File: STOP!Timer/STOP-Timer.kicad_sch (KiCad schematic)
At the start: 18 parts, among them J1 Foot Switch Jack, J4 RJ45, SW1 SW_Push, SW2 SW_Push, SW3 SW_Push, SW4 SW_SPDT, SW5 SW_SPDT

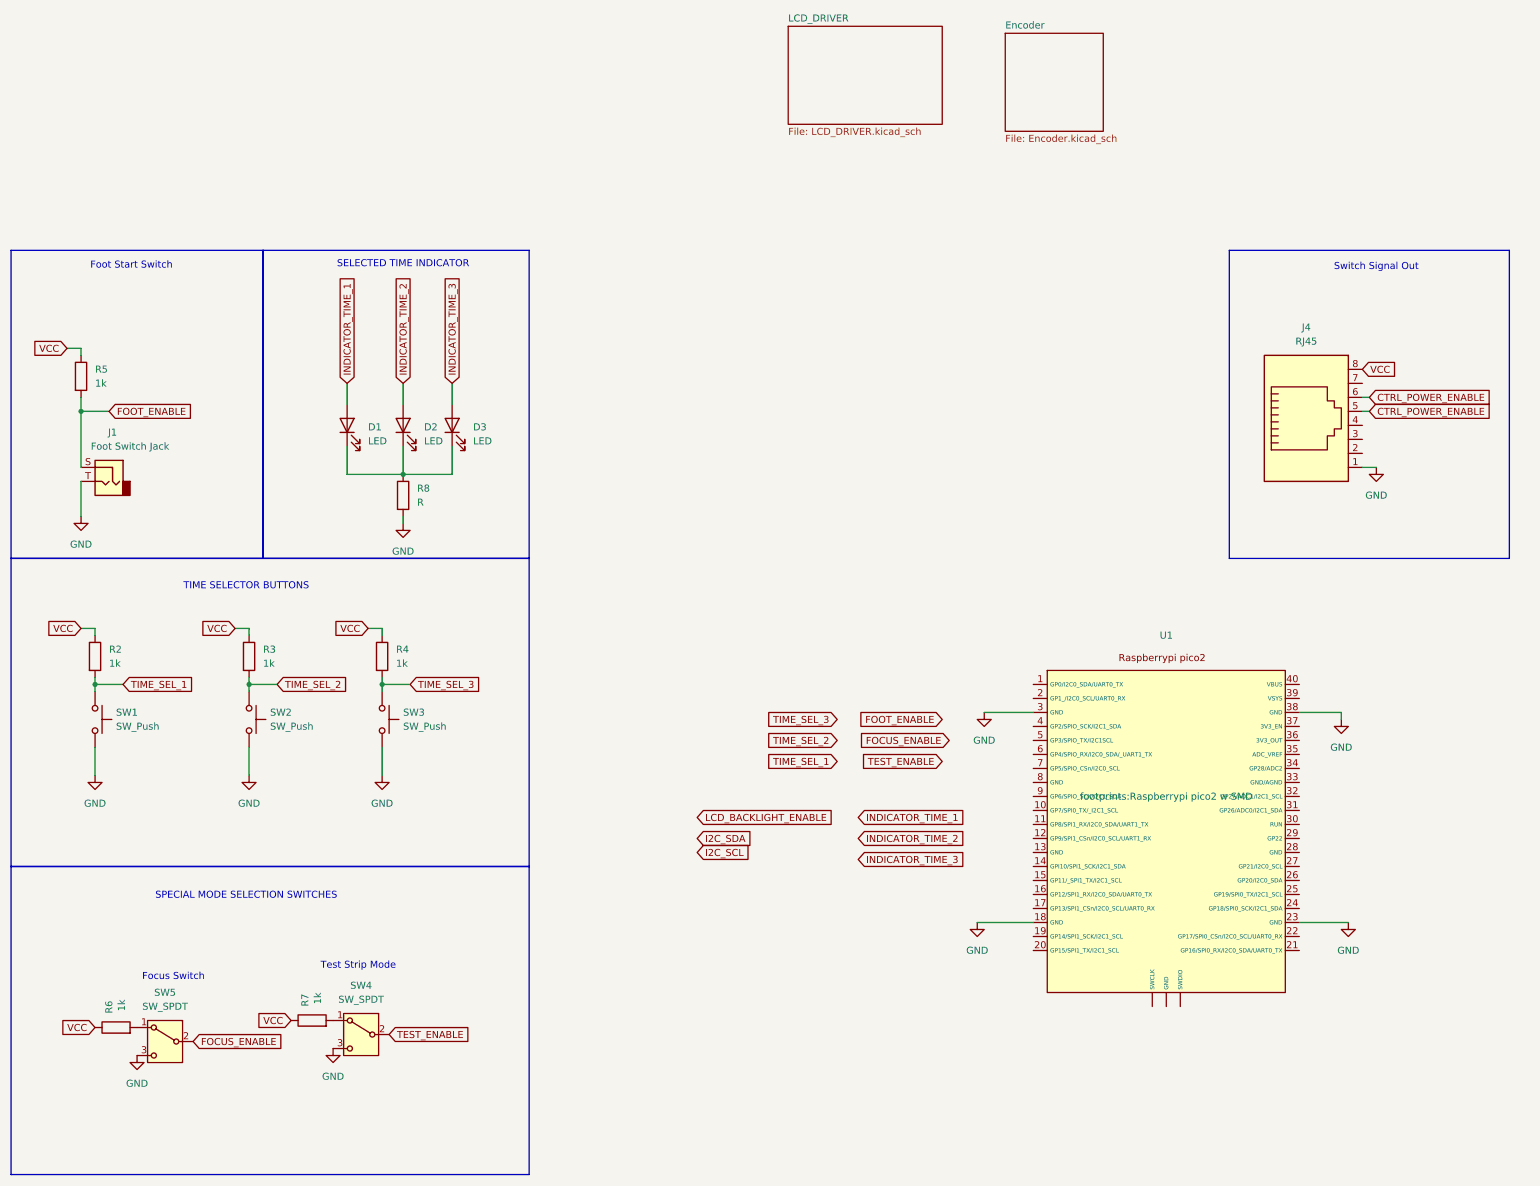
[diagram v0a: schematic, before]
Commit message: Update Schematic
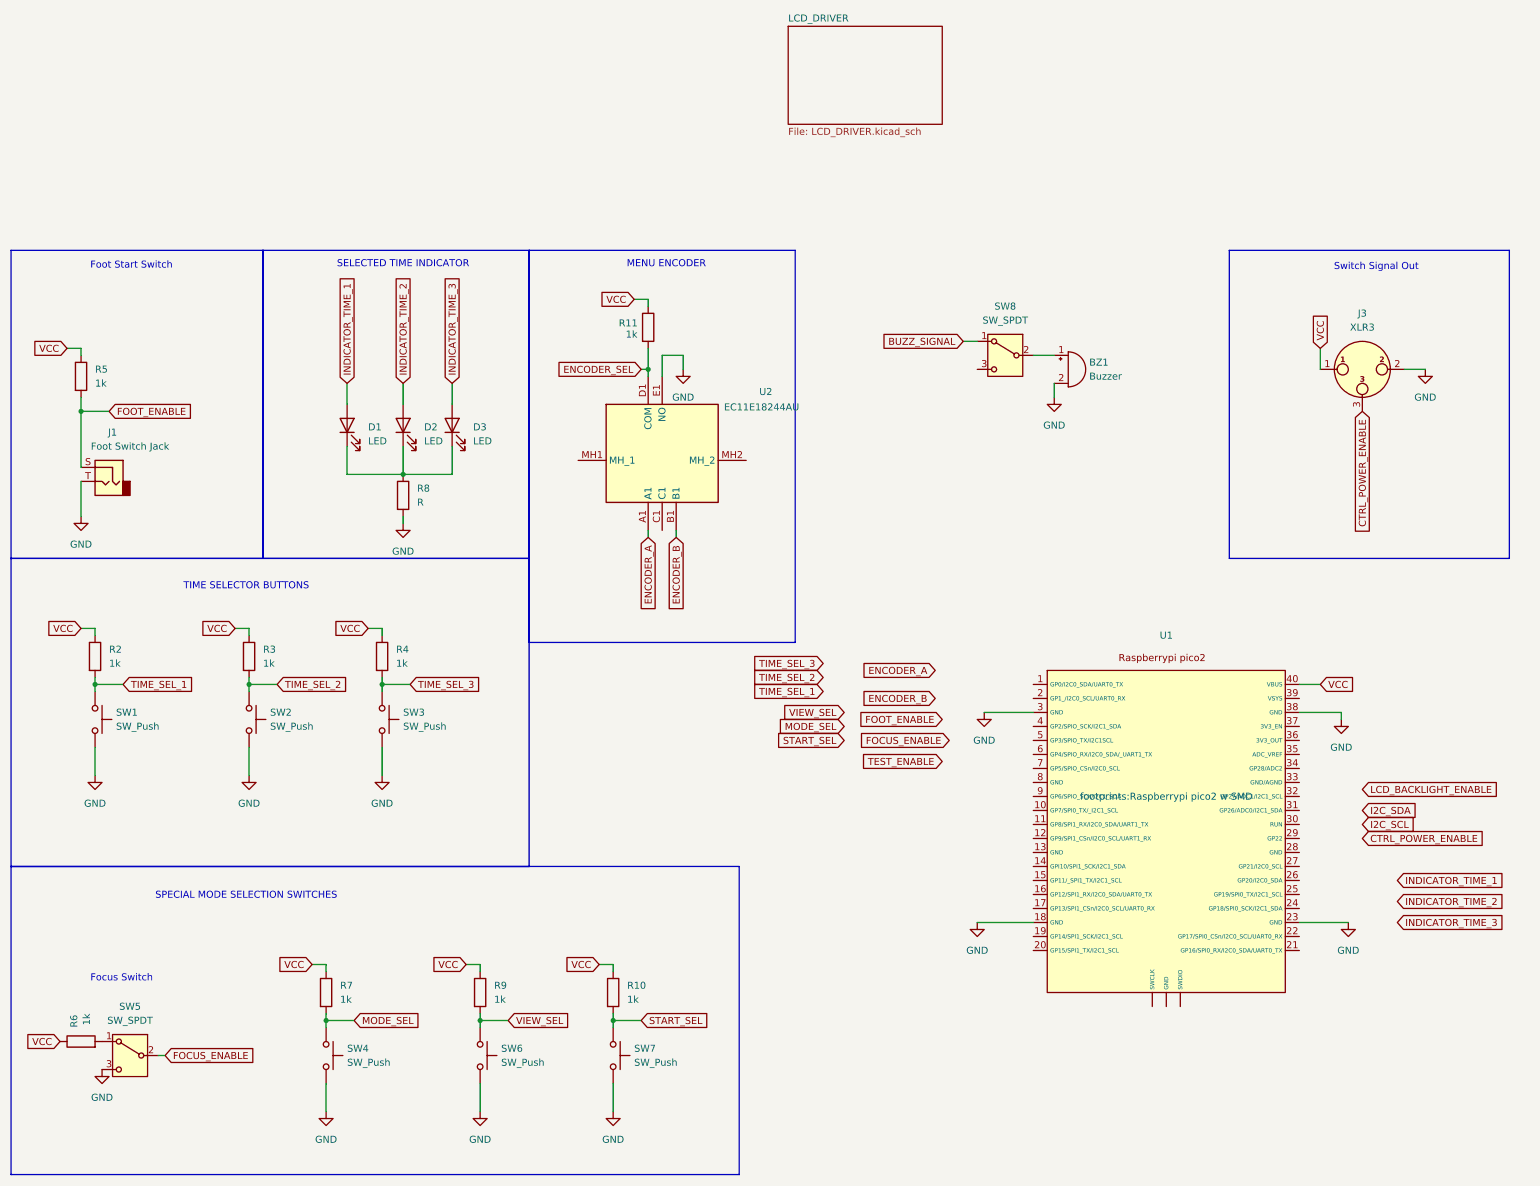
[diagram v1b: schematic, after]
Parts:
- removed J4: RJ45, symbol Connector:RJ45
- removed SW4: SW_SPDT, symbol Switch:SW_SPDT
- added BZ1: Buzzer, Buzzer_Beeper:Buzzer_12x9.5RM7.6, symbol Device:Buzzer
- added J3: XLR3, Connector_Audio:Jack_XLR_Neutrik_NC3FAAH-0_Horizontal, symbol Connector_Audio:XLR3
- added R10, R11, R9: 1k, Resistor_SMD:R_0805_2012Metric_Pad1.20x1.40mm_HandSolder, symbol Device:R
- added SW4, SW6, SW7: SW_Push, Button_Switch_Keyboard:SW_Cherry_MX_1.50u_PCB, symbol Switch:SW_Push
- added SW8: SW_SPDT, symbol Switch:SW_SPDT
- added U2: EC11E18244AU, Rotary_Encoder:RotaryEncoder_Alps_EC11E-Switch_Vertical_H20mm, symbol project:EC11E18244AU
- D1, D2, D3: footprint (none) -> LED_SMD:LED_0805_2012Metric_Pad1.15x1.40mm_HandSolder
- J1: footprint (none) -> Connector_Audio:Jack_6.35mm_Neutrik_NMJ4HCD2_Horizontal
- R2, R3, R4, R5, R6, R7, R8: footprint (none) -> Resistor_SMD:R_0805_2012Metric_Pad1.20x1.40mm_HandSolder
- SW1, SW2, SW3: footprint (none) -> Button_Switch_Keyboard:SW_Cherry_MX_1.50u_PCB; JLC (none) -> C49234237
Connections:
- net CTRL_POWER_ENABLE: now also J3.3
- net GND: now also BZ1.2 (-), J3.2, SW4.2, SW6.2, SW7.2, U2.E1 (NO)
- net VCC: now also U1.40 (VBUS), J3.1, R10.1, R11.1, R9.1
- net MODE_SEL: now reaches R7.2
- net MODE_SEL: now also SW4.1
- new net: BZ1.1 (+), SW8.2 (B)
- new net BUZZ_SIGNAL: SW8.1 (A)
- new net ENCODER_A: U2.A1
- new net ENCODER_B: U2.B1
- new net ENCODER_SEL: R11.2, U2.D1 (COM)
- new net START_SEL: R10.2, SW7.1
- new net VIEW_SEL: R9.2, SW6.1
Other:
- removed sheet Encoder
- note added: "MENU ENCODER"
- note removed: "Test Strip Mode"
- moved on the sheet: R6, SW5
